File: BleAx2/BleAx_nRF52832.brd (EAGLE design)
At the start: 51.7 x 22.9 mm, 60 parts, among them CN1 6p-2.54, J1 2.0MM-90D, J5 MICROUSB, Q1 32MHz, Q2 32MHz, U1 NRF52832, U2 MCP73832T-2ACI/OT-SOT23-5, U4 MIC5225-3.3, X2 32.768kHz

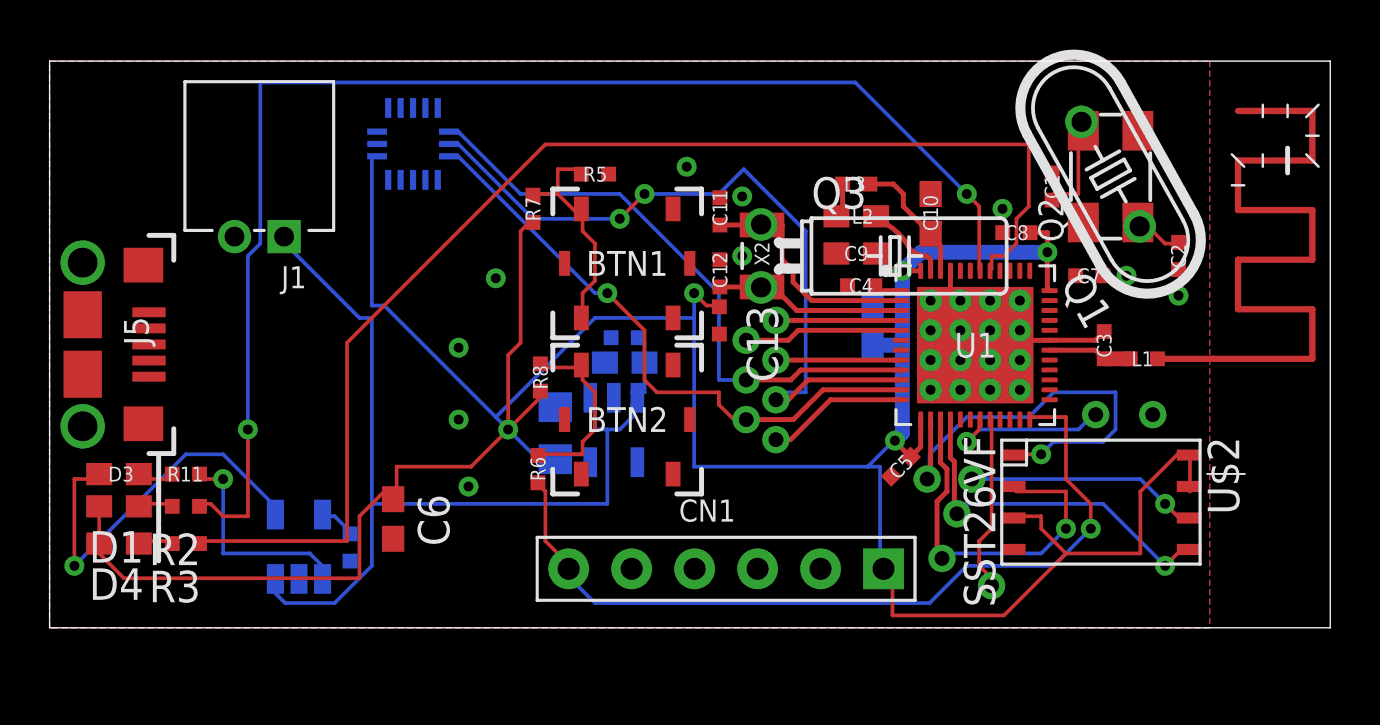
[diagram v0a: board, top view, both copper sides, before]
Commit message: size decrise
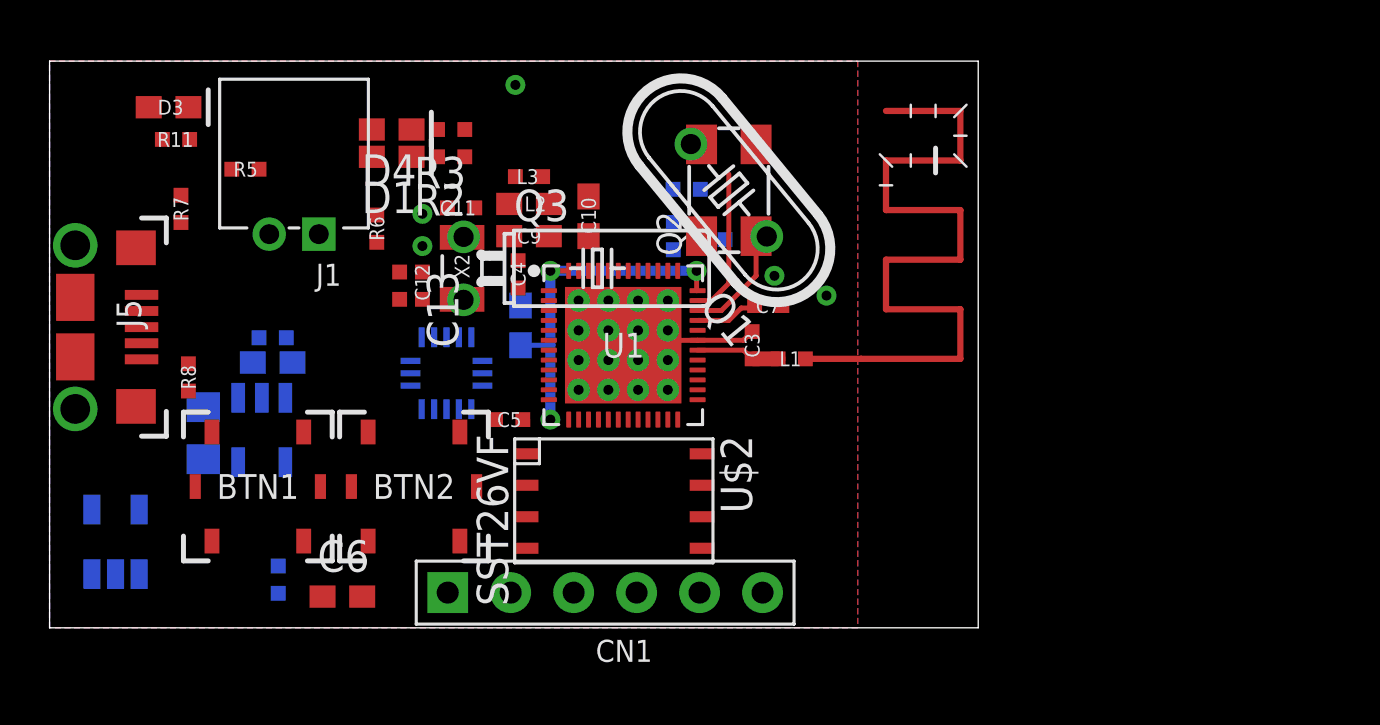
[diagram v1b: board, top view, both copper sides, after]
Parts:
- removed U$1, U$11, U$12, U$13, U$14, U$15, U$16, U$17, U$3, U$4, U$5, U$6, U$7, U$8: 1,1/0,6, wirepad:1,1/0,6
- moved D4 20.0 mm to (13.8, 20.1)
- moved R3 19.8 mm to (16.2, 20.1)
- moved U$2 19.7 mm to (22.9, 5.05)
- moved C2 18.9 mm to (26.7, 15.7), flipped to the bottom, turned to 0 degrees
- moved D1 17.9 mm to (13.8, 19.0)
- moved R2 17.7 mm to (16.2, 19.0)
- moved BTN1 17.4 mm to (8.40, 5.70)
- moved C5 15.9 mm to (18.5, 8.40), turned to 180.1 degrees
- moved Q1 15.4 mm to (27.4, 17.6), turned to 129.4 degrees
- moved Q2 15.4 mm to (27.4, 17.6)
- moved D3 14.9 mm to (4.80, 21.0)
- moved C1 14.7 mm to (25.7, 17.7), flipped to the bottom, turned to 0 degrees
- moved C18 14.2 mm to (19.0, 12.2)
- moved U1 14.2 mm to (23.1, 11.4)
- moved R8 14.2 mm to (5.60, 10.1)
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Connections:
- removed net N$13: U$12.P$1, U1.19
- removed net N$14: U$13.P$1, U1.20
- removed net N$15: U$7.P$1, U1.4
- removed net N$16: U$8.P$1, U1.5
- removed net N$8: U$11.P$1, U1.18
- net LIS_CS: no longer U$3.P$1
- net LIS_INT1: no longer U$1.P$1
- net MISO_01: no longer U$4.P$1
- net MISO_02: now also U1.14; no longer U$14.P$1, U1.15
- net MOSI_01: no longer U$5.P$1
- net MOSI_02: no longer U$16.P$1
- net SCK_01: no longer U$6.P$1
- net SCK_02: no longer U$17.P$1
- net SST26_CE: now also U1.15; no longer U$15.P$1, U1.14
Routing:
- net VDD_P3V3: track 132.5 -> 14.7 mm, vias 5 -> 3
- net LED_01: track 53.7 -> 0.00 mm, vias 2 -> 0
- net LED_02: track 51.0 -> 0.00 mm
- net VDD_BATT: track 39.9 -> 0.00 mm
- net P0.21/RESET: track 34.2 -> 0.00 mm, vias 1 -> 0
- net MISO_01: track 30.7 -> 0.00 mm, vias 2 -> 0
- net LIS_CS: track 25.1 -> 0.00 mm, vias 1 -> 0
- net MOSI_01: track 24.6 -> 0.00 mm
- net SST26_CE: track 18.1 -> 0.00 mm, vias 1 -> 0
- net VCC_P5V0_USB: track 15.8 -> 0.00 mm, vias 1 -> 0
- net MISO_02: track 15.3 -> 0.00 mm, vias 1 -> 0
- net MOSI_02: track 15.1 -> 0.00 mm, vias 1 -> 0
- net XL1: track 11.0 -> 0.00 mm
- net N$7: track 9.54 -> 0.00 mm
- net SCK_02: track 9.40 -> 0.00 mm, vias 1 -> 0
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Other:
- board size 51.7 x 22.9 mm -> 37.5 x 22.9 mm
